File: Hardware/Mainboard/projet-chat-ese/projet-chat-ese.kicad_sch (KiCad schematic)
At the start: 4 parts

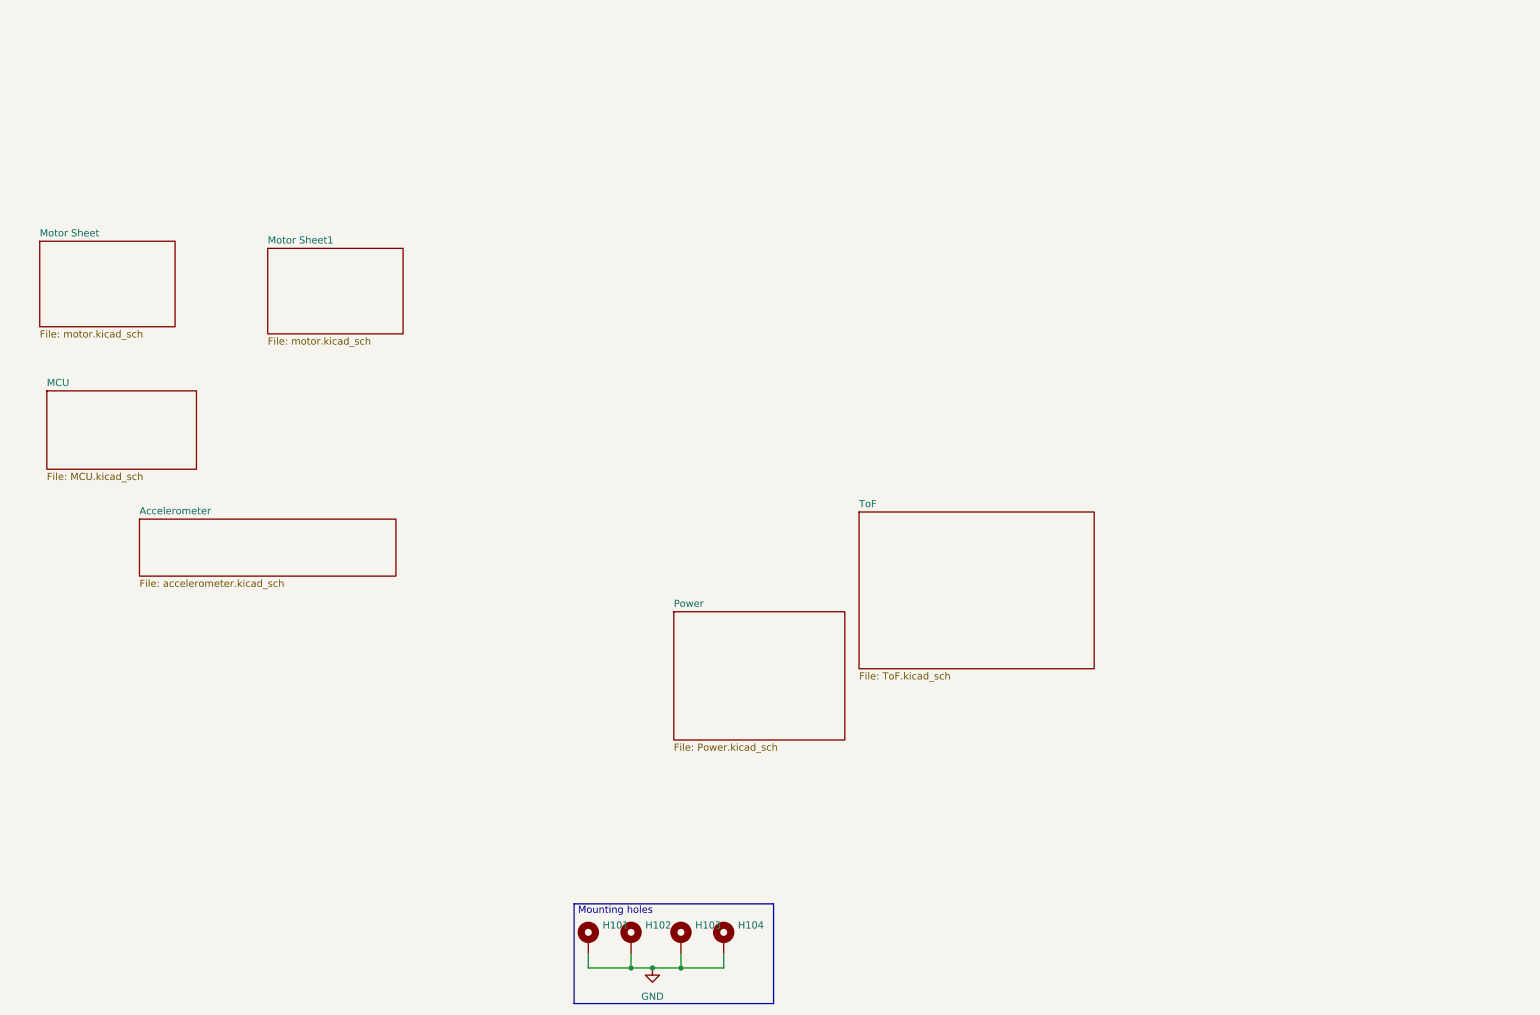
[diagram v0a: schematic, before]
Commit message: [Update] PCB
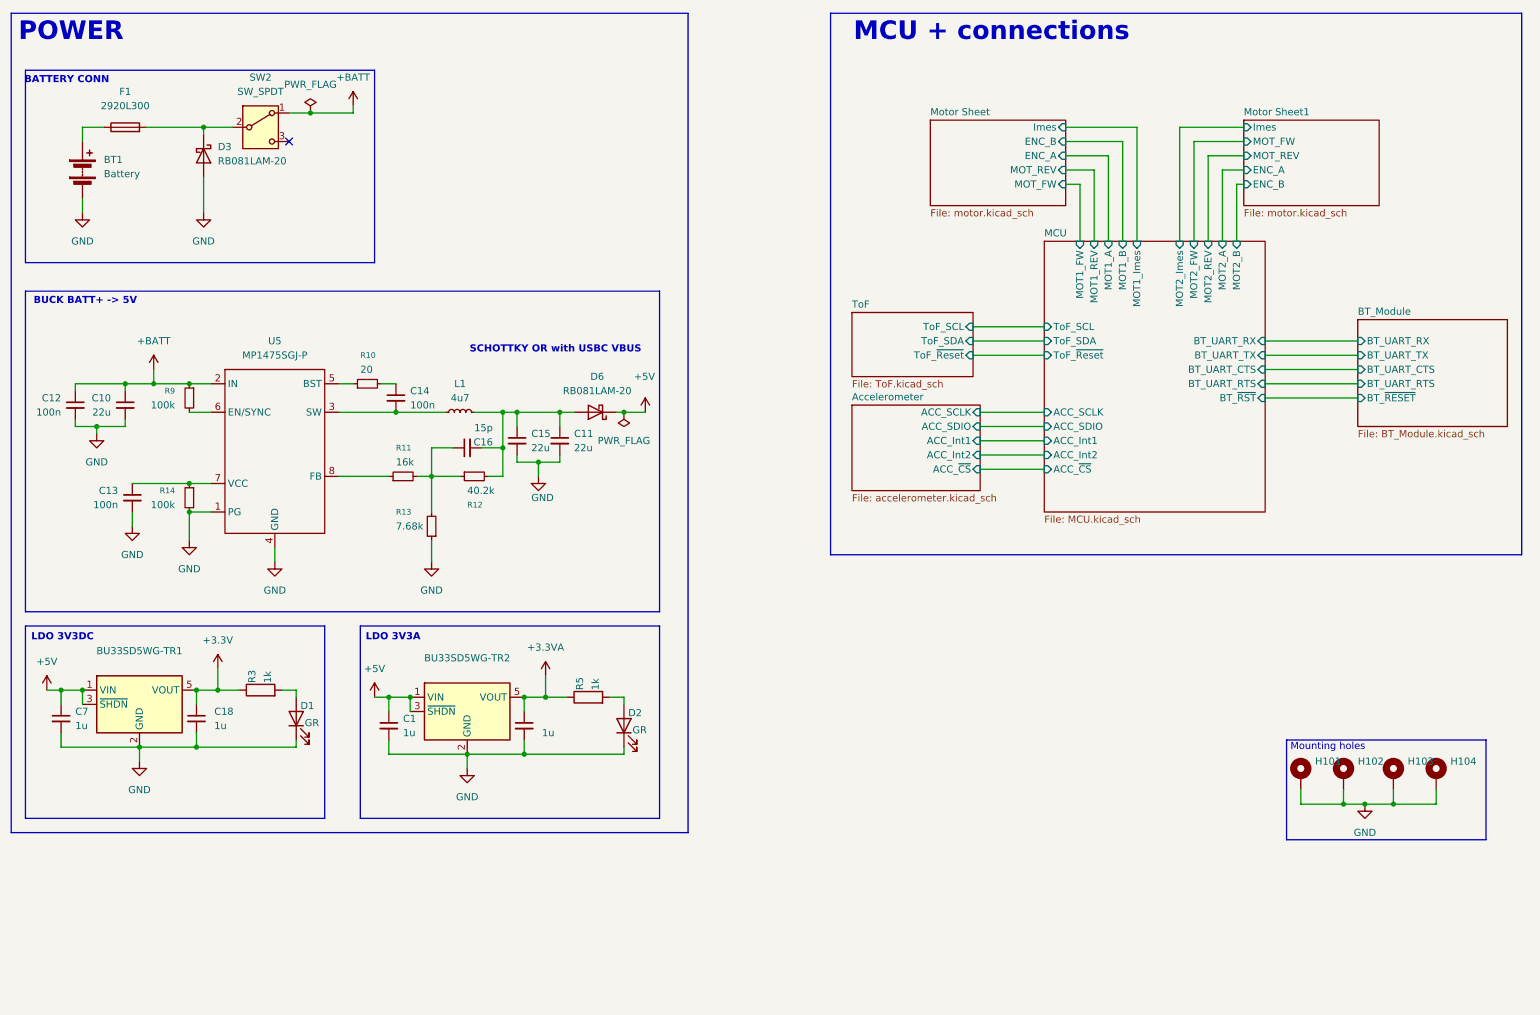
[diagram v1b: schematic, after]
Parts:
- added BT1: Battery, Connector_AMASS:AMASS_XT30U-F_1x02_P5.0mm_Vertical, symbol Device:Battery
- added BU33SD5WG-TR1, BU33SD5WG-TR2: LM1117DT-3.3, Package_TO_SOT_SMD:SOT-23-5, symbol Regulator_Linear:MCP1802x-xx02xOT
- added C1, C18, C2, C7: 1u, Capacitor_SMD:C_0603_1608Metric_Pad1.08x0.95mm_HandSolder, symbol Device:C_Small
- added C10, C11, C15: 22u, Capacitor_SMD:C_0805_2012Metric, symbol Device:C_Small
- added C12, C13, C14: 100n, Capacitor_SMD:C_0402_1005Metric, symbol Device:C_Small
- added C16: 15p, Capacitor_SMD:C_0402_1005Metric, symbol Device:C_Small
- added D1, D2: GR, LED_SMD:LED_0603_1608Metric, symbol Device:LED
- added D3, D6: RB081LAM-20, Diode_SMD:D_SOD-128, symbol Device:D_Schottky
- added F1: 2920L300, symbol Device:Fuse
- added L1: 4u7, symbol Device:L_Small
- added R10: 20, Resistor_SMD:R_0402_1005Metric, symbol Device:R_Small
- added R11: 16k, Resistor_SMD:R_0402_1005Metric, symbol Device:R_Small
- added R12: 40.2k, Resistor_SMD:R_0402_1005Metric, symbol Device:R_Small
- added R13: 7.68k, Resistor_SMD:R_0402_1005Metric, symbol Device:R_Small
- added R14, R9: 100k, Resistor_SMD:R_0402_1005Metric, symbol Device:R_Small
- added R3, R5: 1k, Resistor_SMD:R_0402_1005Metric, symbol Device:R
- added SW2: SW_SPDT, symbol Switch:SW_SPDT
- added U5: MP1475SGJ-P, Package_TO_SOT_SMD:TSOT-23-8, symbol CustomSymbols:MP1475S
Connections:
- net GND: now also BT1.1 (-), BU33SD5WG-TR1.2 (GND), BU33SD5WG-TR2.2 (GND), C1.2, C10.2, C11.2, C12.2, C13.2, C15.2, C18.2, C2.2, C7.2, D1.1 (K), D2.1 (K), D3.2 (A), R13.1, R14.2, U5.1 (PG), U5.4 (GND)
- new net: D1.2 (A), R3.2
- new net: C11.1, C15.1, C16.2, D6.2 (A), L1.1, R12.2
- new net: C14.2, L1.2, U5.3 (SW)
- new net: R9.2, U5.6 (EN/SYNC)
- new net: C13.1, R14.1, U5.7 (VCC)
- new net: C14.1, R10.2
- new net: D3.1 (K), F1.2, SW2.2 (B)
- new net: R10.1, U5.5 (BST)
- new net: R11.1, U5.8 (FB)
- new net: BT1.2 (+), F1.1
- new net: D2.2 (A), R5.2
- new net: C16.1, R11.2, R12.1, R13.2
- new net +3.3V: BU33SD5WG-TR1.5 (VOUT), C18.1, R3.1
- new net +3.3VA: BU33SD5WG-TR2.5 (VOUT), C2.1, R5.1
- new net +5V: BU33SD5WG-TR1.1 (VIN), BU33SD5WG-TR1.3 (~{SHDN}), BU33SD5WG-TR2.1 (VIN), BU33SD5WG-TR2.3 (~{SHDN}), C1.1, C7.1, D6.1 (K)
- new net +BATT: C10.1, C12.1, R9.1, SW2.1 (A), U5.2 (IN)
- no-connect marks 0 -> 1
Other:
- removed sheet Power
- added sheet BT_Module (BT_Module.kicad_sch)
- sheet Accelerometer ports: added ACC_Int1, ACC_Int2, ACC_SCLK, ACC_SDIO, ACC_~{CS}; removed none
- sheet MCU ports: added ACC_Int1, ACC_Int2, ACC_SCLK, ACC_SDIO, ACC_~{CS}, BT_UART_CTS, BT_UART_RTS, BT_UART_RX, BT_UART_TX, BT_~{RST}, MOT1_A, MOT1_B, MOT1_FW, MOT1_Imes, MOT1_REV, MOT2_A, MOT2_B, MOT2_FW, MOT2_Imes, MOT2_REV, ToF_SCL, ToF_SDA, ToF_~{Reset}; removed none
- sheet Motor Sheet ports: added ENC_A, ENC_B, Imes, MOT_FW, MOT_REV; removed none
- sheet Motor Sheet1 ports: added ENC_A, ENC_B, Imes, MOT_FW, MOT_REV; removed none
- sheet ToF ports: added ToF_SCL, ToF_SDA, ToF_~{Reset}; removed none
- note added: "BATTERY CONN"
- note added: "BUCK BATT+ -> 5V"
- note added: "LDO 3V3A"
- note added: "LDO 3V3DC"
- note added: "MCU + connections"
- note added: "POWER"
- note added: "SCHOTTKY OR with USBC VBUS"
- moved on the sheet: H101, H102, H103, H104
